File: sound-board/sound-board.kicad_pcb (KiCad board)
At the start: 2 copper layers, 189.2 x 79.4 mm, 74 parts, among them J1 EXP, J2 EXP, J3 LINE OUT, U1 74HC138, U10 74HC573, U11 74HC283, U12 74HC283, U13 74HC283, U14 74HC283, U15 74HC573, U16 74HC573, U17 74HC273, U18 74HC273, U19 74HC573, U2 74AHC04, U20 74HC283, U21 74HC283, U22 74HC283, U23 74HC283, U24 LM358, U3 74HC138, U4 74HC573, U5 74HC163, U6 74HC573, U7 74HC573, U8 74HC273, U9 74HC273, X1 1MHz

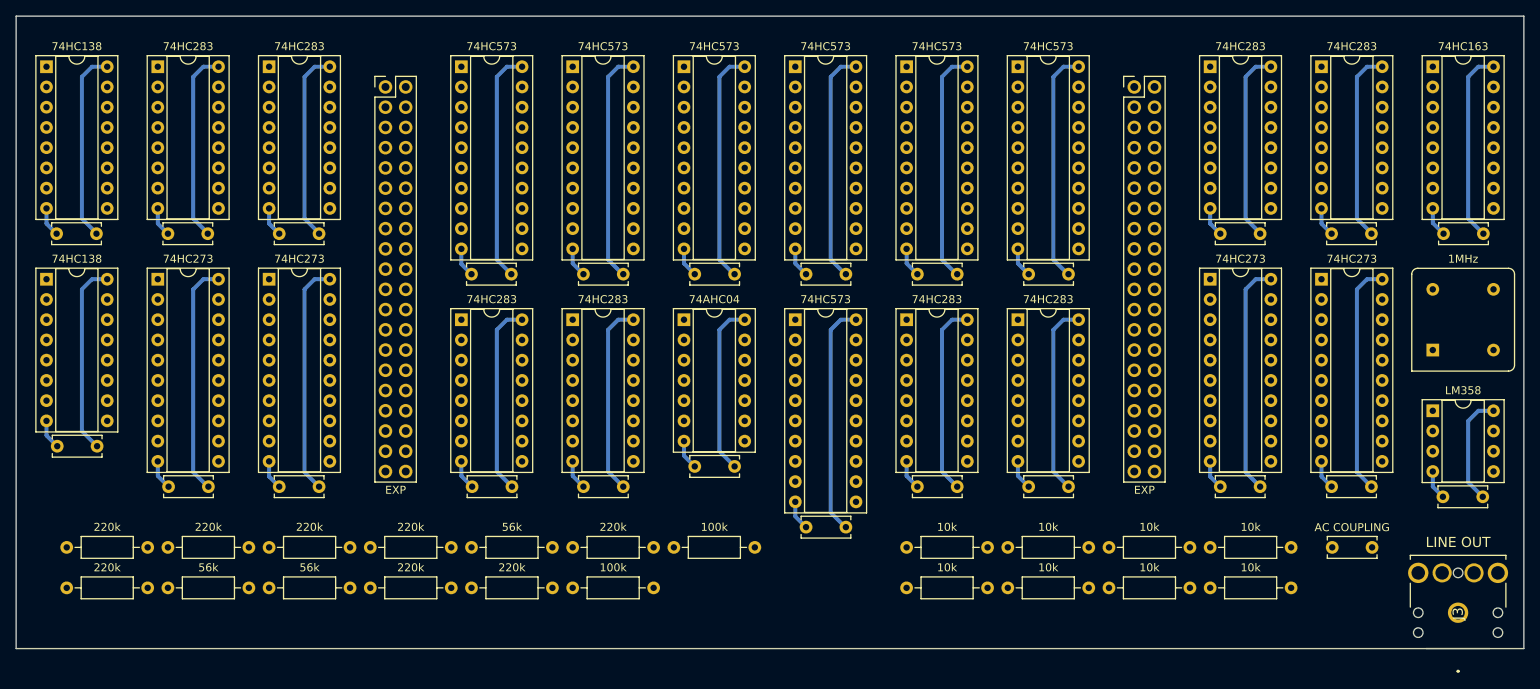
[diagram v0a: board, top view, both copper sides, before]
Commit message: route sound board
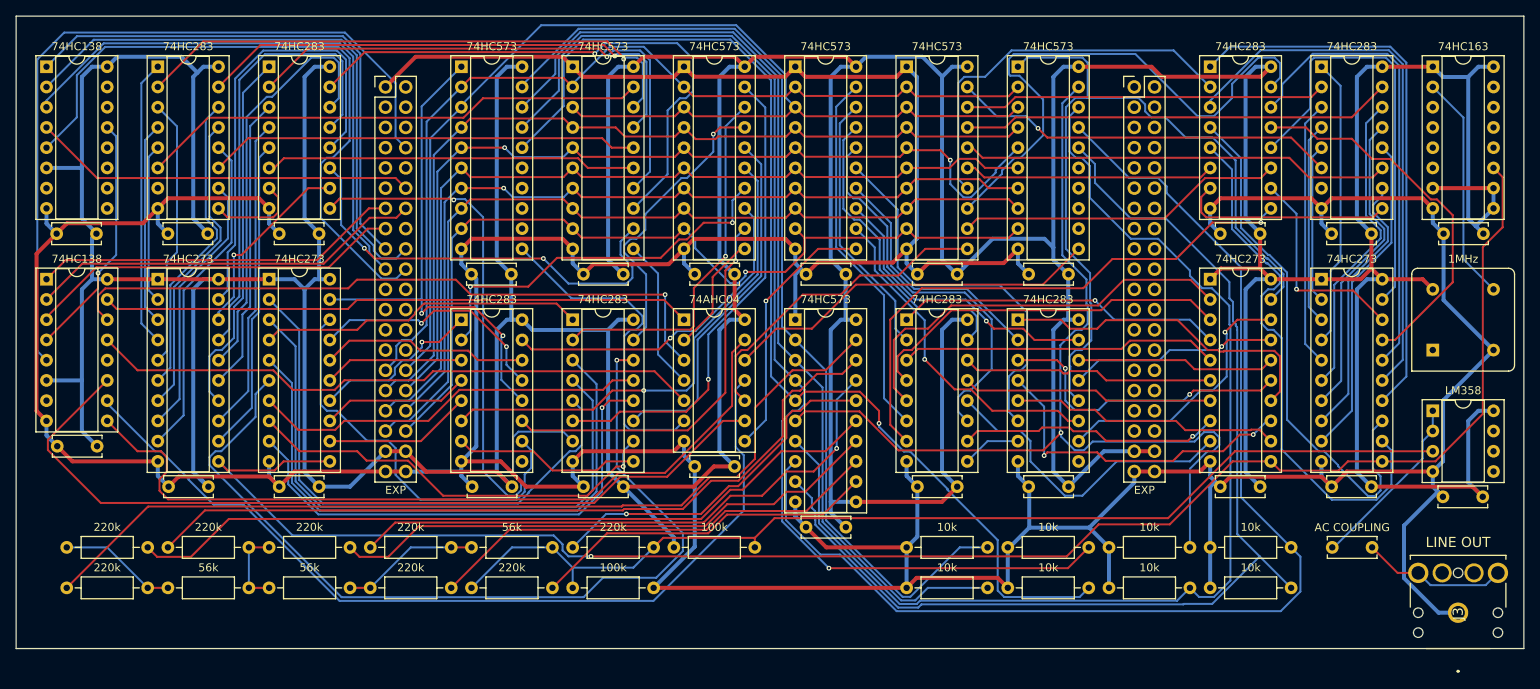
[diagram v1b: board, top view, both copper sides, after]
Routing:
- net GND: track 89.3 -> 692.9 mm
- net +5V: track 623.0 -> 961.4 mm
- net CLK_62K5: track 0.00 -> 219.7 mm, vias 0 -> 1
- net DIGITAL_B_2: track 0.00 -> 150.1 mm
- net D1: track 0.00 -> 147.8 mm
- net DIGITAL_A_2: track 0.00 -> 141.7 mm, vias 0 -> 1
- net DIGITAL_B_1: track 0.00 -> 140.9 mm
- net DIGITAL_B_3: track 0.00 -> 138.1 mm
- net DIGITAL_A_3: track 0.00 -> 137.3 mm, vias 0 -> 1
- net ANALOG_OUT: track 0.00 -> 133.6 mm
- net DIGITAL_A_1: track 0.00 -> 123.2 mm
- net DIGITAL_A_0: track 0.00 -> 123.1 mm
- net DIGITAL_B_0: track 0.00 -> 122.3 mm, vias 0 -> 1
- net D0: track 0.00 -> 118.3 mm
- net BUFFERED_A_0: track 0.00 -> 115.7 mm
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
